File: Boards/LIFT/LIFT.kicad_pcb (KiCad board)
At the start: 4 copper layers, 58 x 82.5 mm, 11 parts, among them J1 Screw_Terminal_01x02, J2 393570004, J3 393570004, J4 393570004, J5 Screw_Terminal_01x02, U3 MAX485_MODULE_5V_LOGIC_TLL_TO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

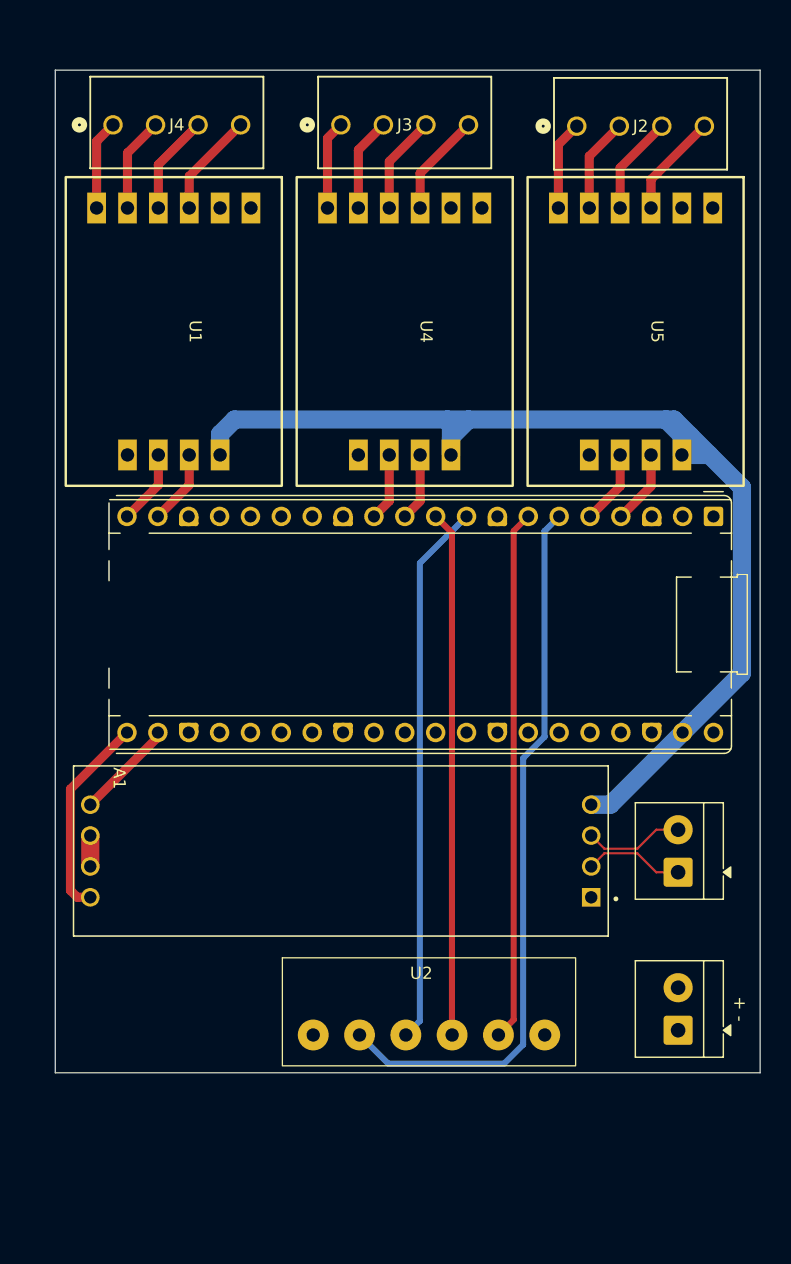
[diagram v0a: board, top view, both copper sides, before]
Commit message: PCB Loadcells
Agora sim acho que ta acabado
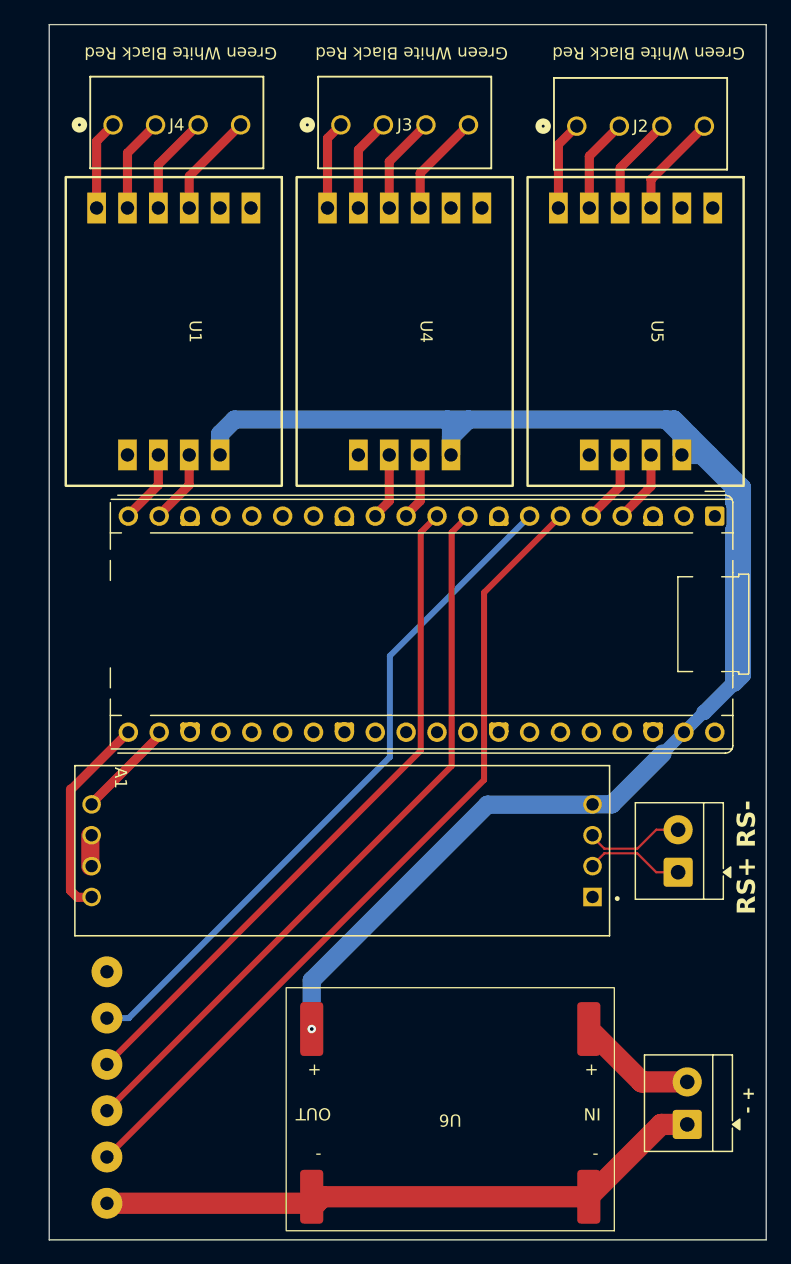
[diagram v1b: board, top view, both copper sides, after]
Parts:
- added G***: LOGO, FEUP-text:Feup-text, B.Cu at (158.0, 144.5)
- added U6: ~, DCDCModule:DCDC_Module, F.Cu at (155.0, 137.9)
- U2: moved to B.Cu
- moved U2 22.2 mm to (134.4, 136.3), turned to 90 degrees
- moved J1 7.79 mm to (174.5, 138.8)
- moved A1 0.11 mm to (176.8, 88.7)
- moved U3 0.11 mm to (146.1, 116.2)
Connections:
- J1 pad 2: /3V3 -> /V_In
- J3 pad 3: /A1+ -> /A1-
- J3 pad 4: /A1- -> /A1+
- J4 pad 3: /A3+ -> /A3-
- J4 pad 4: /A3- -> /A3+
- U1 pad 3: /A3+ -> /A3-
- U1 pad 4: /A3- -> /A3+
- U4 pad 3: /A1+ -> /A1-
- U4 pad 4: /A1- -> /A1+
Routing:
- net /5V: track 92.6 -> 164.9 mm, vias 0 -> 1
- net GND: track 0.00 -> 51.3 mm
- net /SD_CLK: track 44.7 -> 61.2 mm
- net /SD_MOSI: track 43.2 -> 56.4 mm
- net /SD_CS: track 43.7 -> 56.8 mm
- net /V_In: track 0.00 -> 9.90 mm
- net /SD_MISO: track 59.8 -> 68.3 mm
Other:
- board size 58 x 82.5 mm -> 59 x 100 mm
- board text added: "Green White Black Red"
- board text added: "LIFT"
- board text added: "RS+ RS-"
